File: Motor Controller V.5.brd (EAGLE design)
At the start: 153.7 x 59.4 mm, 54 parts, among them IC1 MEGA8-P, J1 NMJ6HCD2-RM, Q1 IRF540

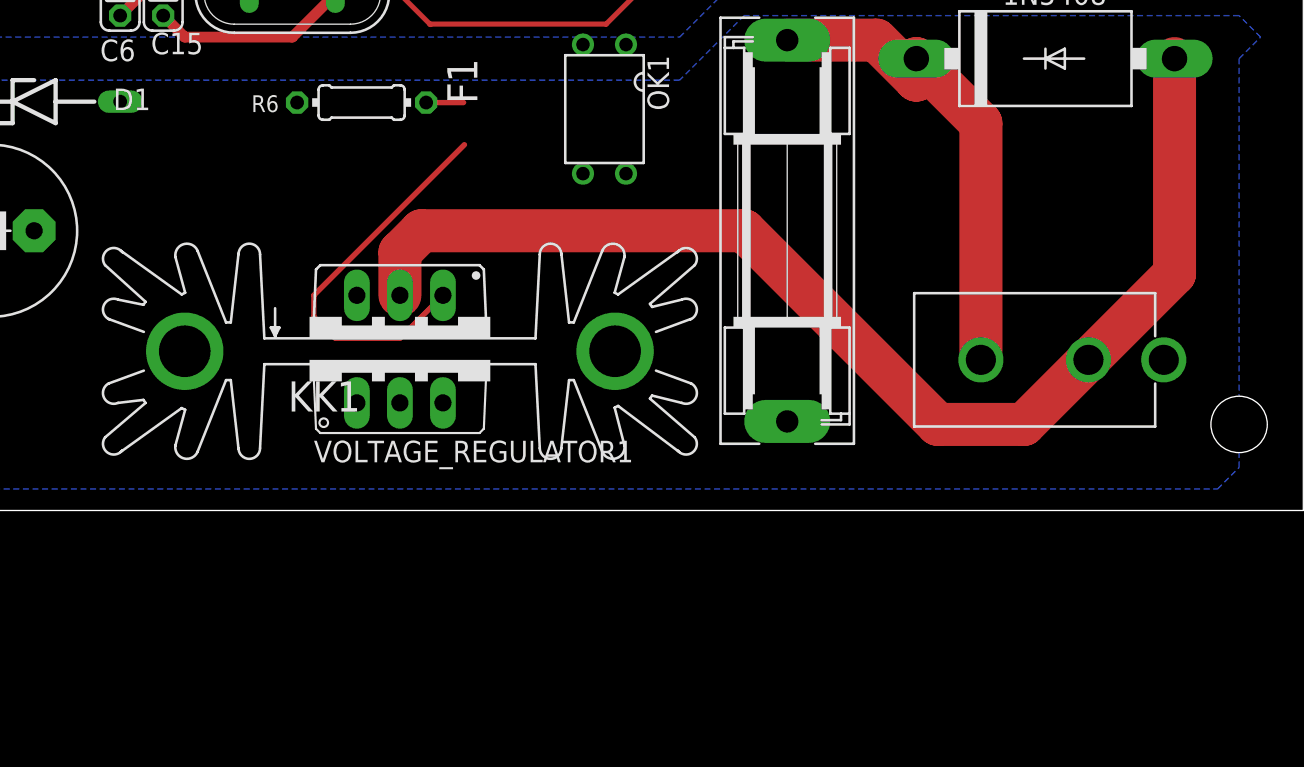
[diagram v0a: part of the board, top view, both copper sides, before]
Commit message: Starting to route on new board with updated components. v5.1
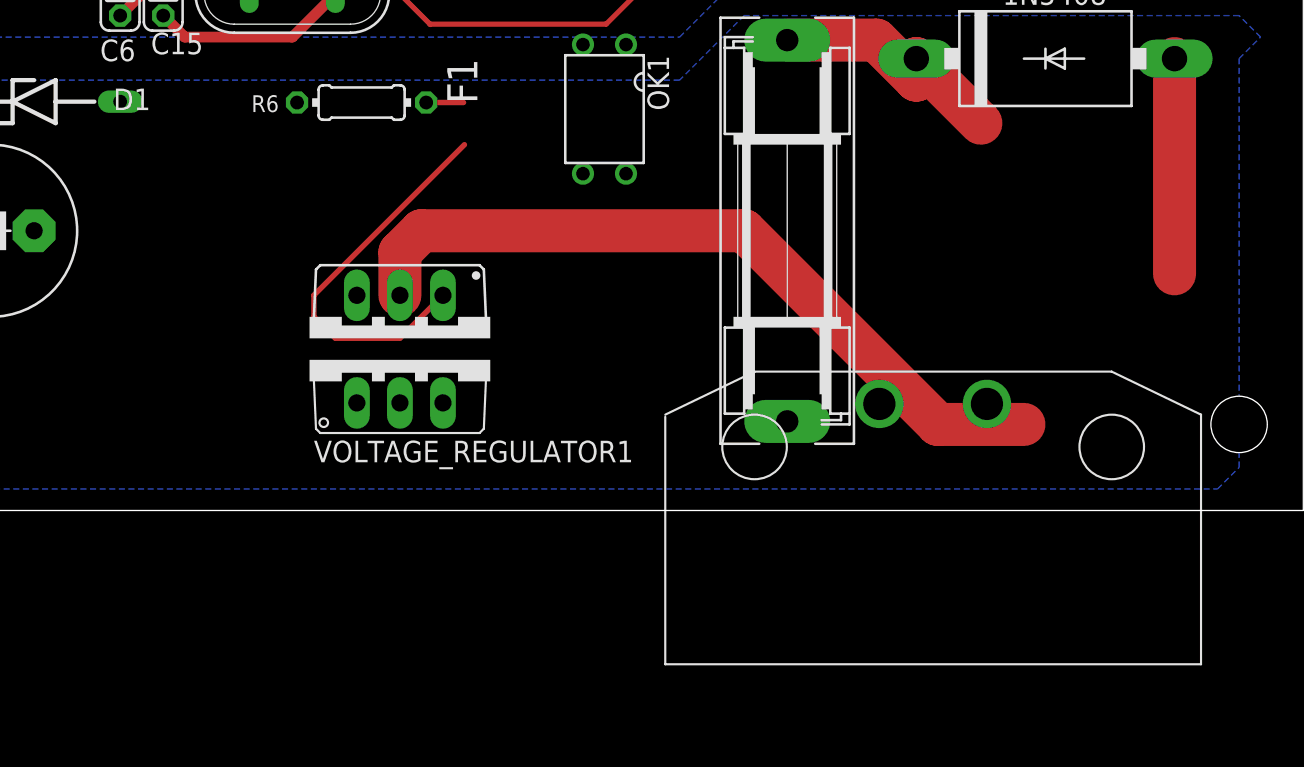
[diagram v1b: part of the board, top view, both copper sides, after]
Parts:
- removed KK1: SK104, Benson Motor Controller:SK104
- MOTOR_CONNECTOR: value 641963-1 -> MATE-N-LOK_193839-1; device Benson:641963-1_TYC -> Benson Motor Controller:MATE-N-LOK_2PIN_CONNECTOR
- moved MOTOR_CONNECTOR 10.5 mm to (131.8, 1.21)
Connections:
- net MOTOR+: now also MOTOR_CONNECTOR.P$1; no longer MOTOR_CONNECTOR.2
- net MOTOR-: now also MOTOR_CONNECTOR.P$2; no longer MOTOR_CONNECTOR.1
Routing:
- net MOTOR+: track 29.2 -> 15.3 mm
- net MOTOR-: track 69.9 -> 57.3 mm
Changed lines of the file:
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@@
 <attribute name="VALUE" x="139.205" y="38.105" size="1.27" layer="27" rot="R90" align="center"/>
-</element>
-<element name="KK1" library="Benson Motor Controller" package="SK104" package3d_urn="urn:adsk.eagle:package:14176/1" value="SK104" x="100.33" y="7.62" smashed="yes">
-<attribute name="MF" value="" x="100.33" y="7.62" size="1.778" layer="27" display="off"/>
-<attribute name="MPN" value="" x="100.33" y="7.62" size="1.778" layer="27" display="off"/>
-<attribute name="NAME" x="93.726" y="3.302" size="1.778" layer="25" ratio="10"/>
-<attribute name="OC_NEWARK" value="unknown" x="100.33" y="7.62" size="1.778" layer="27" display="off"/>
-<attribute name="POPULARITY" value="2" x="180.34" y="-25.4" size="1.778" layer="27" display="off"/>
 </element>
 <element name="L2" library="Benson Motor Controller" package="RCP1317_INDUCTOR" value="1.2mH (min 0.4A max 4Ohm)" x="30.48" y="19.05" smashed="yes" rot="R270">
@@
 <attribute name="VALUE" x="54.5592" y="51.1048" size="1.27" layer="27" ratio="10"/>
 </element>
-<element name="MOTOR_CONNECTOR" library="Benson" package="641963-1_TYC" value="641963-1" x="140.97" y="6.35" smashed="yes" rot="R180">
-<attribute name="BUILT_BY" value="EMA_UL_Team" x="107.95" y="95.25" size="1.778" layer="27" rot="R180" display="off"/>
-<attribute name="MANUFACTURER_PART_NUMBER" value="641963-1" x="107.95" y="95.25" size="1.778" layer="27" rot="R180" display="off"/>
-<attribute name="MF" value="" x="140.97" y="6.35" size="1.778" layer="27" rot="R180" display="off"/>
-<attribute name="MPN" value="" x="140.97" y="6.35" size="1.778" layer="27" rot="R180" display="off"/>
-<attribute name="OC_NEWARK" value="unknown" x="140.97" y="6.35" size="1.778" layer="27" rot="R180" display="off"/>
-<attribute name="SOURCELIBRARY" value="Tyco_2012-04-26" x="107.95" y="95.25" size="1.778" layer="27" rot="R180" display="off"/>
-<attribute name="VENDOR" value="TE Connectivity" x="107.95" y="95.25" size="1.778" layer="27" rot="R180" display="off"/>
+<element name="MOTOR_CONNECTOR" library="Benson Motor Controller" package="MATE-N-LOK_2PIN_CONNECTOR" value="MATE-N-LOK_193839-1" x="131.8021125" y="1.210353125" smashed="yes" rot="R180">
+<attribute name="MF" value="" x="131.8021125" y="1.210353125" size="1.778" layer="27" rot="R180" display="off"/>
+<attribute name="MPN" value="" x="131.8021125" y="1.210353125" size="1.778" layer="27" rot="R180" display="off"/>
+<attribute name="OC_NEWARK" value="unknown" x="131.8021125" y="1.210353125" size="1.778" layer="27" rot="R180" display="off"/>
 </element>
 <element name="PROGRAMMING_HEADER" library="pinhead" library_urn="urn:adsk.eagle:library:325" package="2X03" package3d_urn="urn:adsk.eagle:package:22462/2" value="" x="93.98" y="50.8" smashed="yes">
@@
 <signal name="MOTOR-">
 <contactref element="Q1" pad="D"/>
-<contactref element="MOTOR_CONNECTOR" pad="1"/>
 <contactref element="1N5408" pad="A"/>
 <wire x1="146.05" y1="24.13" x2="146.05" y2="11.43" width="2.54" layer="1"/>
-<wire x1="146.05" y1="11.43" x2="140.97" y2="6.35" width="2.54" layer="1"/>
 <wire x1="100.33" y1="10.16" x2="100.33" y2="12.7" width="2.54" layer="1"/>
 <wire x1="100.33" y1="12.7" x2="101.6" y2="13.97" width="2.54" layer="1"/>
@@
 <wire x1="120.65" y1="13.97" x2="132.08" y2="2.54" width="2.54" layer="1"/>
 <wire x1="132.08" y1="2.54" x2="137.16" y2="2.54" width="2.54" layer="1"/>
-<wire x1="137.16" y1="2.54" x2="140.97" y2="6.35" width="2.54" layer="1"/>
+<contactref element="MOTOR_CONNECTOR" pad="P$2"/>
+<wire x1="128.6271125" y1="3.750353125" x2="146.05" y2="11.43" width="0" layer="19" extent="1-1"/>
+<wire x1="137.16" y1="2.54" x2="128.6271125" y2="3.750353125" width="0" layer="19" extent="1-1"/>
 </signal>
 <signal name="MOTOR+">
 <contactref element="1N5408" pad="C"/>
 <contactref element="F1" pad="1"/>
-<contactref element="MOTOR_CONNECTOR" pad="2"/>
 <wire x1="123.19" y1="25.2222" x2="128.4478" y2="25.2222" width="2.54" layer="1"/>
 <wire x1="128.4478" y1="25.2222" x2="130.81" y2="22.86" width="2.54" layer="1"/>
 <wire x1="130.81" y1="22.86" x2="130.81" y2="24.13" width="2.54" layer="1"/>
 <wire x1="130.81" y1="24.13" x2="134.62" y2="20.32" width="2.54" layer="1"/>
-<wire x1="134.62" y1="20.32" x2="134.62" y2="6.35" width="2.54" layer="1"/>
+<contactref element="MOTOR_CONNECTOR" pad="P$1"/>
+<wire x1="134.62" y1="20.32" x2="134.9771125" y2="3.750353125" width="0" layer="19" extent="1-1"/>
 </signal>
 <signal name="5VHIGHSIDE">
